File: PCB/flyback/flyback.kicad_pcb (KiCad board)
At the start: 2 copper layers, 47 parts, among them Q1 IRFR3410TRLPBF, T1 Transformer_1P_1S, U1 UC3843_SOIC8, U2 4N25, U3 TL431DBZ

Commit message: Layout Update
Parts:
- moved R1 245.8 mm to (36.8, 110.4)
- moved R3 242.8 mm to (30.3, 119.3)
- moved C9 242.5 mm to (37.9, 124.8)
- moved C4 231.3 mm to (38.8, 45.3), turned to 90 degrees
- moved C3 228.7 mm to (50.4, 107.2)
- moved R2 223.5 mm to (44.2, 117.8)
- moved C5 222.9 mm to (57.5, 123.8)
- moved C2 219.6 mm to (50.8, 117.1)
- moved C1 215.7 mm to (47.3, 112.1)
- moved C6 211.6 mm to (49.6, 45.8), turned to 90 degrees
- moved R8 206.3 mm to (108.3, 171.2), turned to 90 degrees
- moved R6 204.6 mm to (58.4, 115.2)
- moved R9 203.8 mm to (92.8, 171.4), turned to 90 degrees
- moved C7 199.8 mm to (46.9, 125.4)
- moved C8 195.1 mm to (43.9, 45.5), turned to 90 degrees
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
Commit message: PCB Update
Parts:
- added R20: 10k, Resistor_SMD:R_0805_2012Metric, F.Cu at (117.1, 91.5)
- D2: moved to B.Cu
- T1: footprint Transformer_THT:Transformer_CHK_EI48-10VA_Neutral -> Transformer_THT:Transformer_CHK_EI48-8VA_Neutral
- moved R10 121.4 mm to (134.9, 82.4), turned to 90 degrees
- moved C11 114.6 mm to (134.9, 87.3), turned to 90 degrees
- moved R4 110.7 mm to (116.1, 64.2), turned to -90 degrees
- moved R5 103.6 mm to (119.8, 64.2), turned to -90 degrees
- moved R11 92.4 mm to (155.2, 115.2), turned to 90 degrees
- moved C4 75.8 mm to (113.2, 60.1), turned to -90 degrees
- moved C8 73.6 mm to (116.1, 59.6), turned to -90 degrees
- moved C6 71.6 mm to (119.8, 60.2), turned to -90 degrees
- moved C7 70.5 mm to (104.8, 85.1), turned to -90 degrees
- moved R13 68.2 mm to (213.5, 97.4), turned to -90 degrees
- moved U1 65.8 mm to (95.3, 87.5)
- moved R9 64.5 mm to (133.6, 121.4), turned to -90 degrees
- moved C5 63.4 mm to (108.1, 85.6), turned to -90 degrees
- moved Q1 63.1 mm to (123.7, 84.0), turned to 90 degrees
- moved R3 62.8 mm to (85.1, 88.5), turned to -90 degrees
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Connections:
- C1 pad 2: GNDA -> GND1
- C10 pad 1: Net-(C10-Pad1) -> /Vin
- C13 pad 1: GNDA -> GND2
- C15 pad 1: GNDA -> GND2
- C16 pad 1: GNDA -> GND2
- C17 pad 1: GNDA -> GND2
- C18 pad 1: GNDA -> GND2
- C19 pad 1: GNDA -> GND2
- C20 pad 1: GNDA -> GND2
- C3 pad 2: GNDA -> GND1
- C4 pad 1: GNDA -> GND1
- C4 pad 2: Net-(C10-Pad1) -> /Vin
- C5 pad 1: GNDA -> GND1
- C5 pad 2: Net-(C10-Pad1) -> /Vin
- C6 pad 1: GNDA -> GND1
- C6 pad 2: Net-(C10-Pad1) -> /Vin
- C7 pad 1: GNDA -> unconnected-(C7-Pad1)
- C7 pad 2: Net-(C10-Pad1) -> /Vin
- C8 pad 1: GNDA -> GND1
- C8 pad 2: Net-(C10-Pad1) -> /Vin
- C9 pad 1: GNDA -> GND1
- R19 pad 2: GNDA -> GND2
- R4 pad 1: Net-(C10-Pad1) -> /Vin
- R5 pad 1: unconnected-(R5-Pad1) -> /Vin
- R7 pad 2: GNDA -> GND1
- R8 pad 2: GNDA -> GND1
- R9 pad 2: GNDA -> GND1
- T1 pad 10: GNDA -> (no net)
- T1 pad 12: (no net) -> GND2
- T1 pad 5: Net-(C10-Pad1) -> (no net)
- T1 pad 6: Net-(D2-Pad2) -> /Vin
- T1 pad 7: (no net) -> Net-(D2-Pad2)
- U1 pad 5: GNDA -> GND1
- U1 pad 7: Net-(C10-Pad1) -> /Vin
- U3 pad 3: GNDA -> GND2
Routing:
- net Net-(C3-Pad1): track 0.00 -> 1.82 mm
- added copper zone on F.Cu, net /Vout

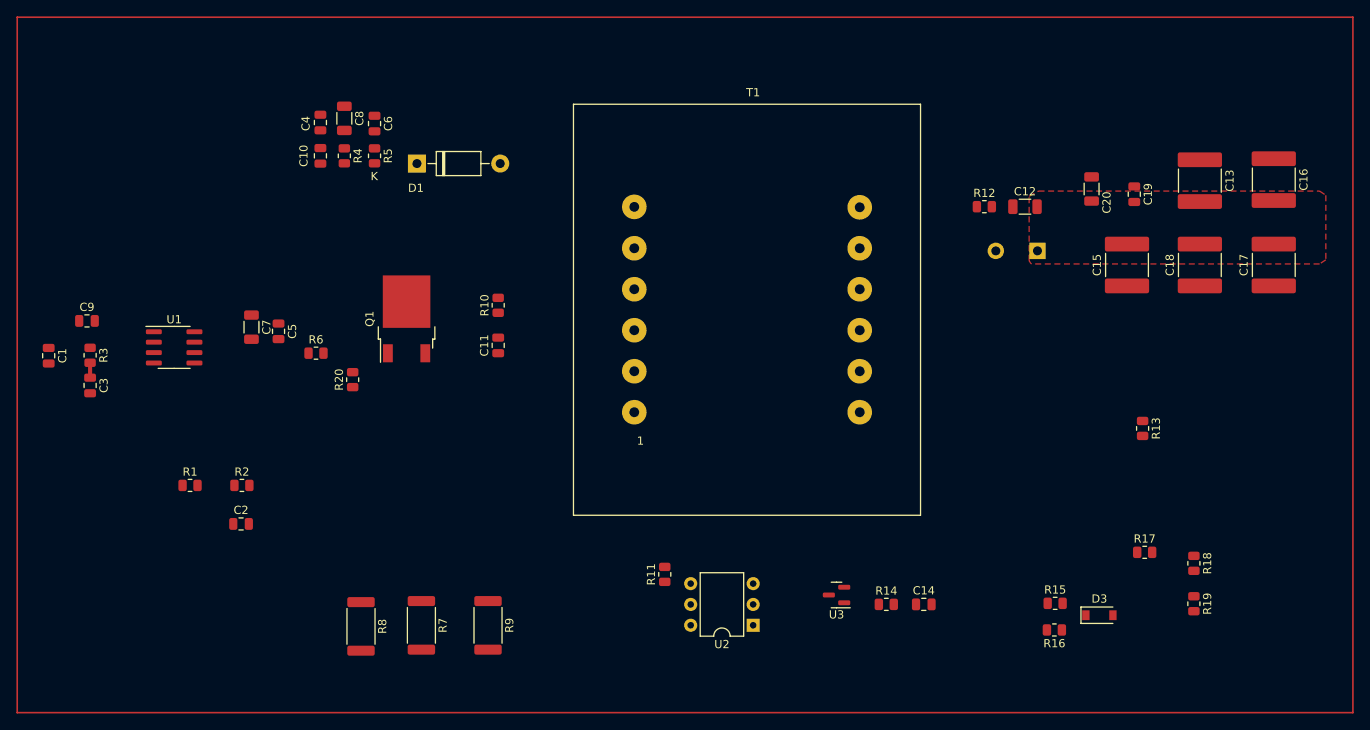
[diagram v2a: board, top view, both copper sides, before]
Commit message: PCB Update
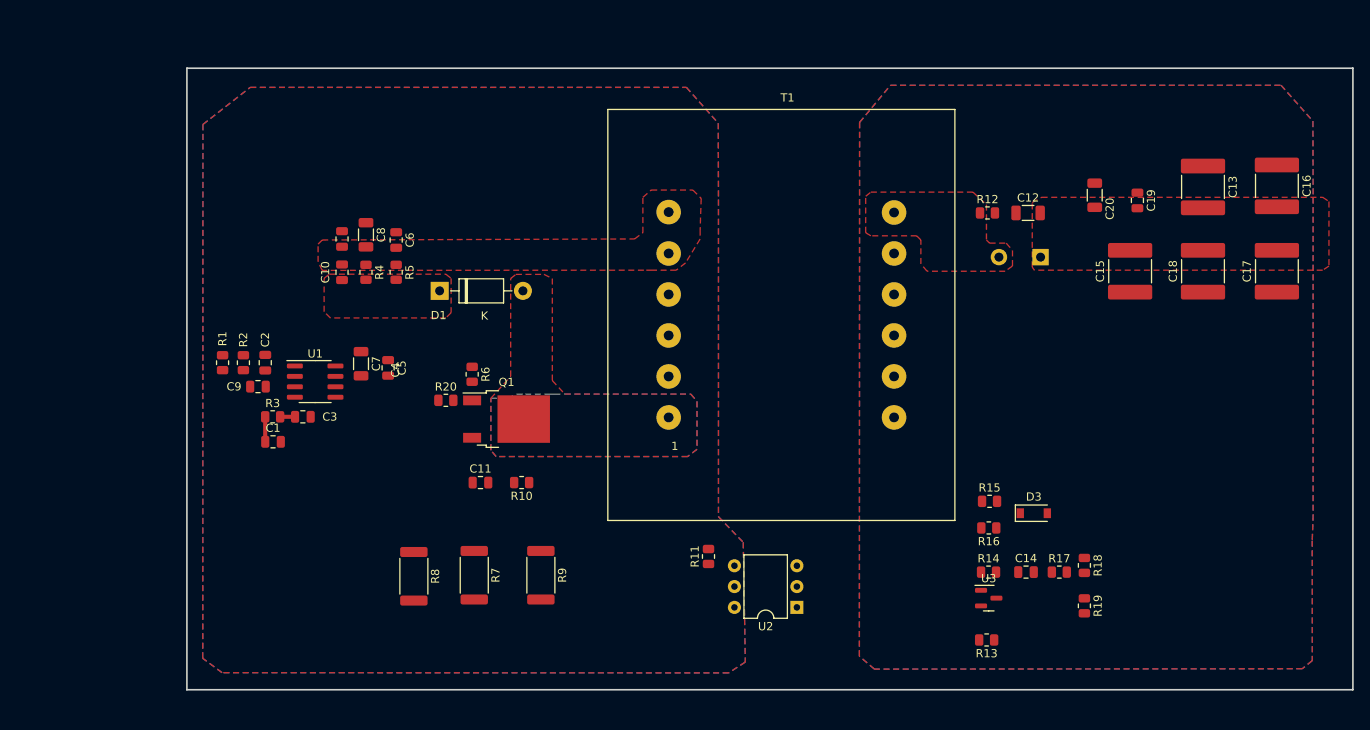
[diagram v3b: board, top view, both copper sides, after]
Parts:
- moved R13 32.1 mm to (194.5, 123.2), turned to 180 degrees
- moved C1 29.3 mm to (107.4, 99.0), turned to 0 degrees
- moved C3 26.2 mm to (111.0, 96.0), turned to 0 degrees
- moved R3 23.5 mm to (107.4, 96.0), turned to 0 degrees
- moved C9 22.3 mm to (105.6, 92.3)
- moved R10 21.8 mm to (137.7, 104.0), turned to 180 degrees
- moved C2 19.9 mm to (106.5, 89.4), turned to 90 degrees
- moved R6 19.2 mm to (131.7, 90.8), turned to -90 degrees
- moved U3 18.6 mm to (194.7, 118.1), turned to 0 degrees
- moved U1 17.7 mm to (112.5, 91.7)
- moved Q1 17.3 mm to (135.9, 96.3), turned to 0 degrees
- moved C11 16.9 mm to (132.7, 104.0), turned to 0 degrees
- moved D1 15.8 mm to (127.7, 80.6)
- moved R1 15.5 mm to (101.3, 89.4), turned to -90 degrees
- moved R2 15.0 mm to (103.8, 89.4), turned to 90 degrees
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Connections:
- C7 pad 1: unconnected-(C7-Pad1) -> GND1
- D3 pad 2: GNDA -> GND2
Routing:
- net /Vref: track 0.00 -> 3.05 mm
- added copper zone on F.Cu, net /Vin
- added copper zone on B.Cu, net GND1
- added copper zone on F.Cu, net GND1
- added copper zone on B.Cu, net GND2
- added copper zone on F.Cu, net GND2
- added copper zone on F.Cu, net Net-(C10-Pad2)
- added copper zone on B.Cu, net Net-(D1-Pad2)
- added copper zone on F.Cu, net Net-(D1-Pad2)
- added copper zone on F.Cu, net Net-(D2-Pad2)
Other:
- board outline added: 142.2 x 75.8 mm
